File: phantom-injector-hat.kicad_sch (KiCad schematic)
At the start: 40 parts, among them J1 Conn_02x20_Odd_Even, J2 Conn_02x03_Top_Bottom, J3 Conn_01x03, J4 Conn_01x03, SW1 SW_SPST, U1 LT8362EMSE-PBF

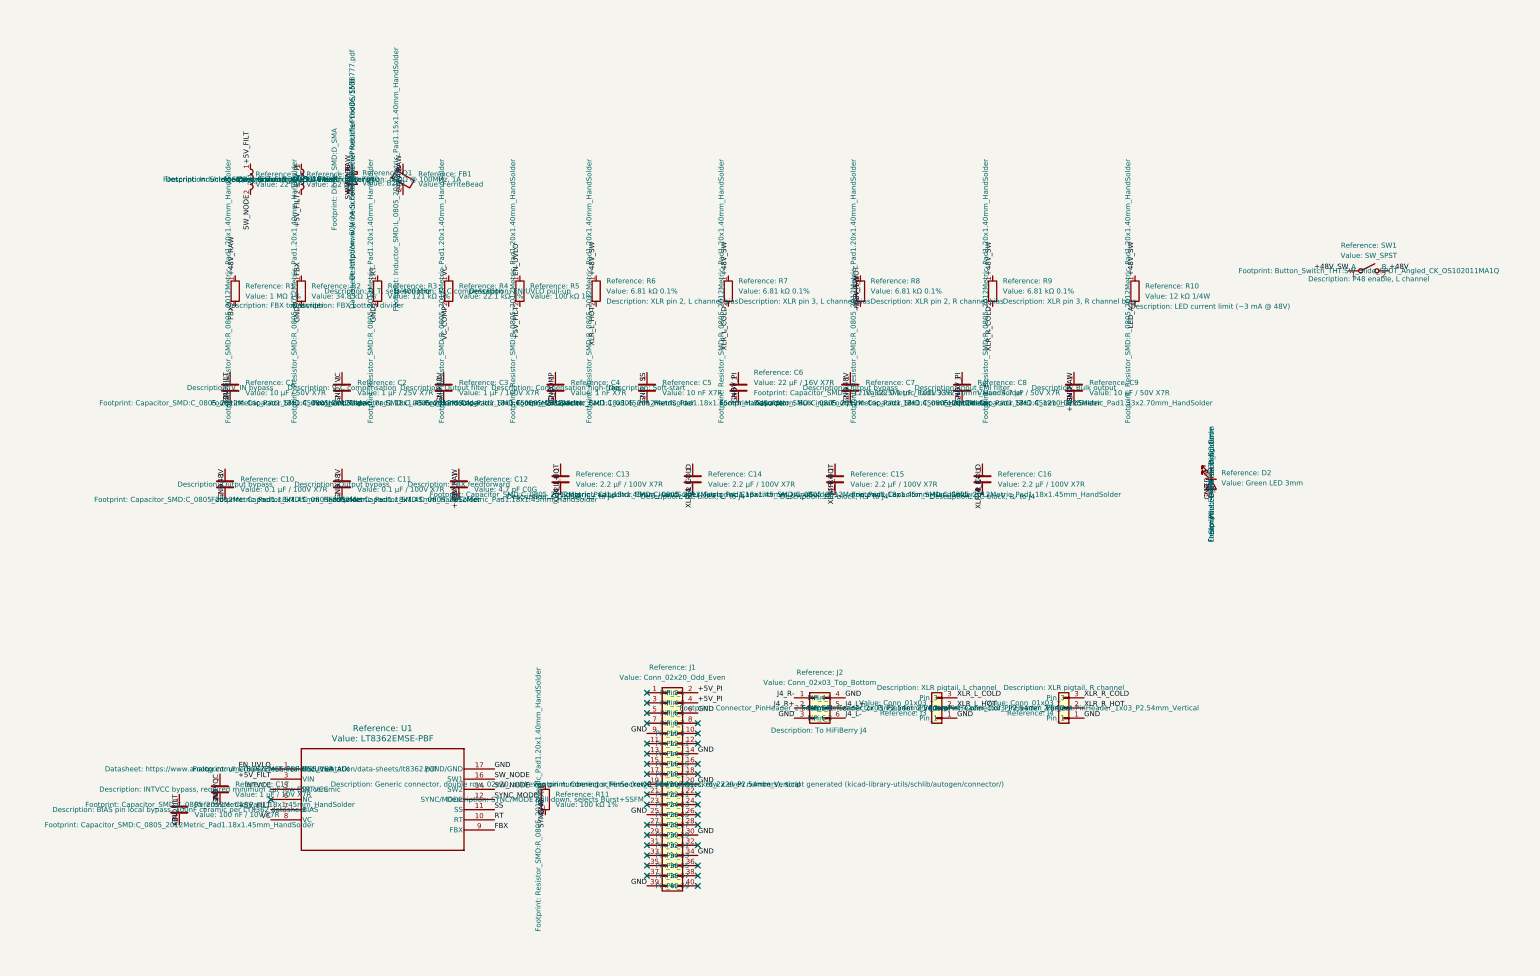
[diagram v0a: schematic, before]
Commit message: checkpoint
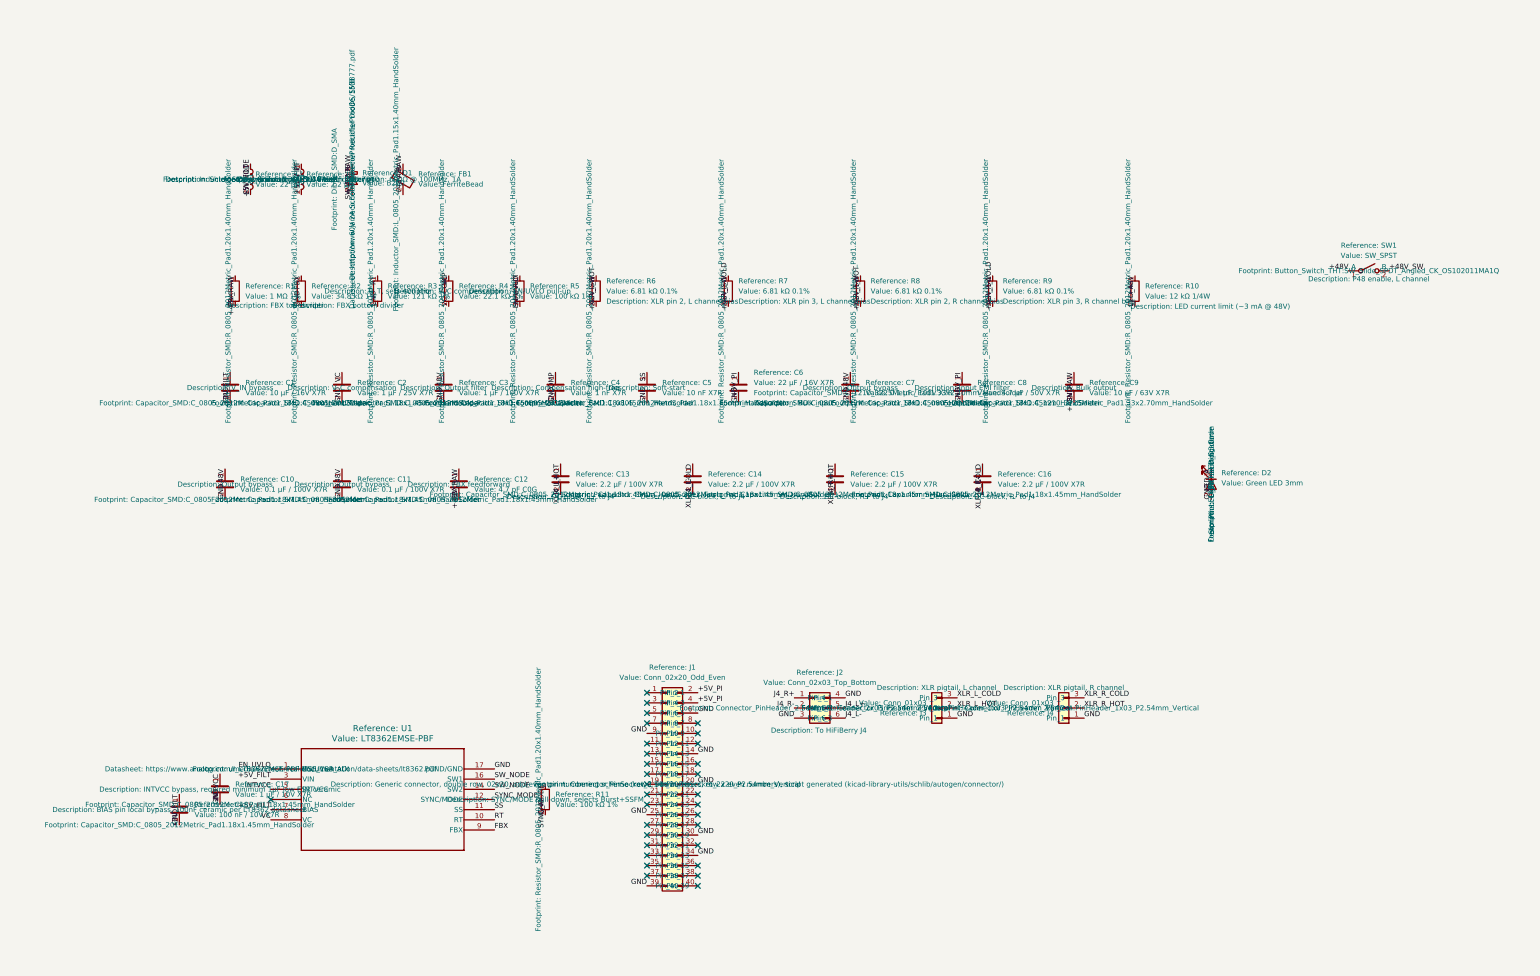
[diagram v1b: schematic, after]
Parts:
- C1: value 10 µF / 50V X7R -> 10 µF / 16V X7R
- C9: value 10 µF / 50V X7R -> 10 µF / 63V X7R
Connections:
- net +48V: now also R10.1, SW1.1 (A); no longer SW1.2 (B)
- net +48V_SW: now also SW1.2 (B); no longer R10.1, SW1.1 (A)
- net J4_R+: now also J2.1 (Pin_1); no longer J2.2 (Pin_2)
- net J4_R-: now also J2.2 (Pin_2); no longer J2.1 (Pin_1)
